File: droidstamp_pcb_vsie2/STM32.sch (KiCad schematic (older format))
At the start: 52 parts, among them P6 CONN_5X2, P8 CONN_12X2, P9 CONN_12X2, Q2 BS170F, Q3 BS170F, Q4 BS170F, Q5 BS170F, Q6 BS170F, Q7 BS170F, Q8 BS170F, Q9 BS170F, U10 STM32F105RC, U11 LT1117CST-3.3, U12 ZXMHC3F381N8, U13 ZXMHC3F381N8, U14 ZXMHC3F381N8, U15 ZXMHC3F381N8, U9 STM32F4_LQFP100, X3 12MHz

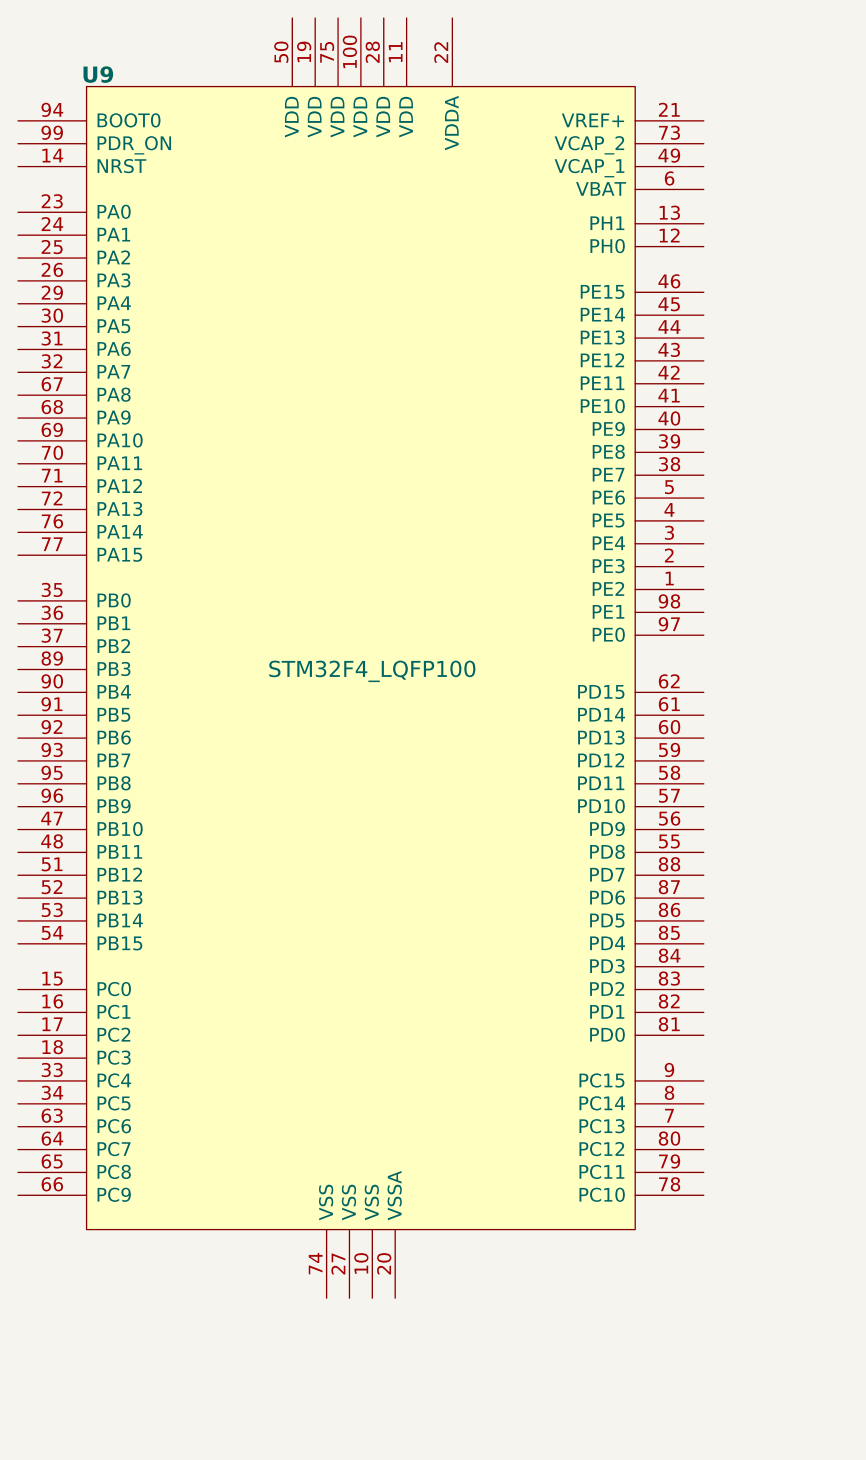
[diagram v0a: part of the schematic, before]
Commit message: sync with las sie_bot_v2
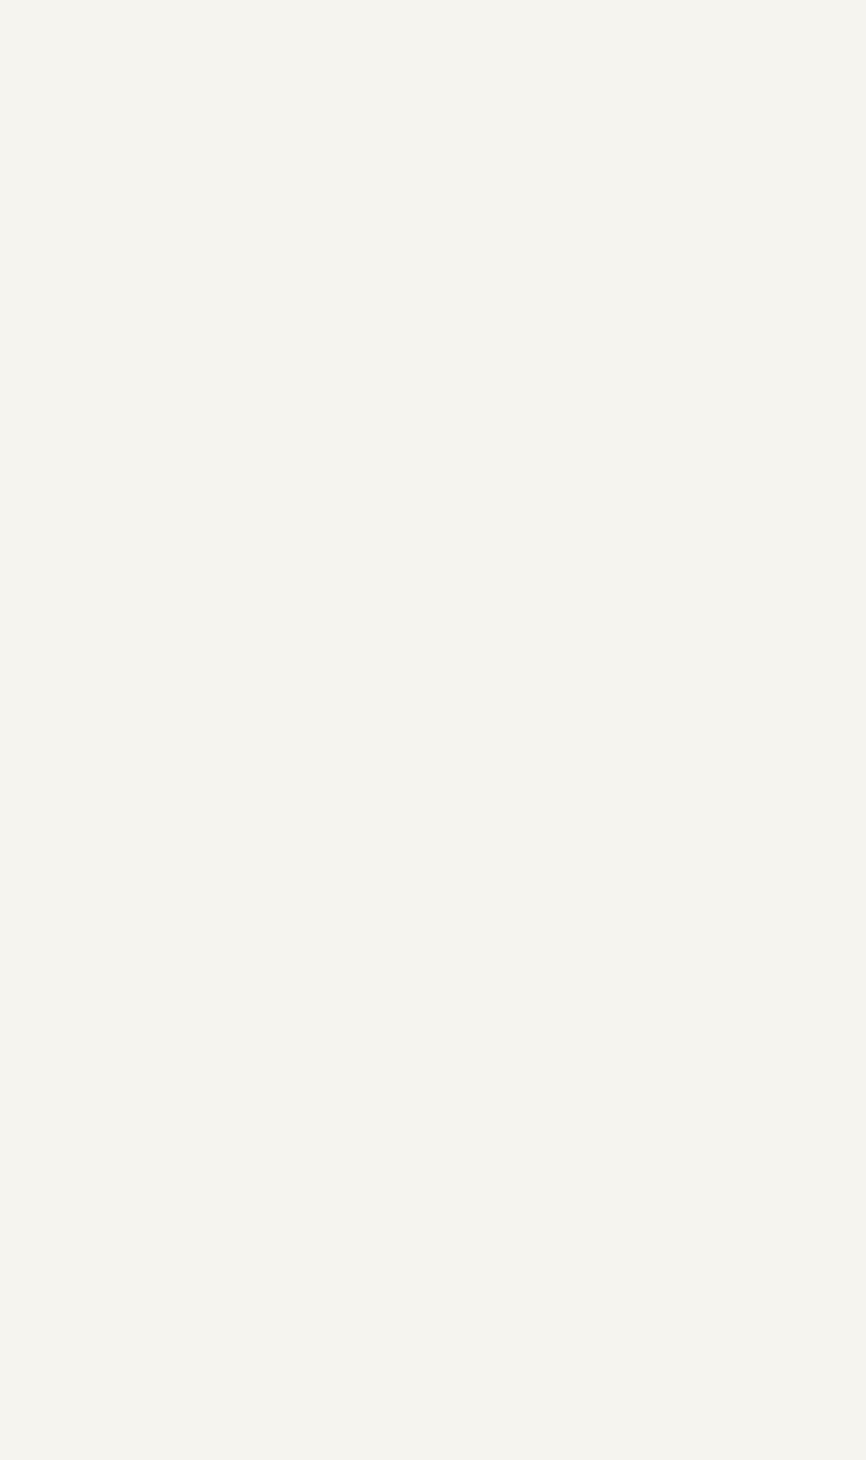
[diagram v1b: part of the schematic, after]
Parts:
- removed U9: STM32F4_LQFP100, TQFP_100, symbol STM32F4_LQFP100
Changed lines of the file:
@@
-EESchema Schematic File Version 2  date Thu 29 Mar 2012 07:34:40 PM COT
+EESchema Schematic File Version 2  date Fri 30 Mar 2012 08:38:46 AM COT
 LIBS:con-jack
 LIBS:adm3101e
@@
 LIBS:lt1117cst
 LIBS:zxmhc3f381n8
-LIBS:stm32f4_lqfp100
 LIBS:i.mx233stamp-cache
 EELAYER 25  0
@@
 $Descr User 12000 10000
 encoding utf-8
-Sheet 4 5
+Sheet 3 5
 Title ""
 Date "30 mar 2012"
@@
 C19, C21 2.2uF para cortex M4\nC19. C21 = Ohms para cortex M3
 $Comp
-L GND #PWR98
+L GND #PWR087
 U 1 1 4F3EDF04
 P 4400 7650
-F 0 "#PWR98" H 4400 7650 30  0001 C CNN
+F 0 "#PWR087" H 4400 7650 30  0001 C CNN
 F 1 "GND" H 4400 7580 30  0001 C CNN
 	1    4400 7650
@@
 $EndComp
 $Comp
-L GND #PWR97
+L GND #PWR088
 U 1 1 4F3EDF01
 P 4200 7650
-F 0 "#PWR97" H 4200 7650 30  0001 C CNN
+F 0 "#PWR088" H 4200 7650 30  0001 C CNN
 F 1 "GND" H 4200 7580 30  0001 C CNN
 	1    4200 7650
@@
 $EndComp
 $Comp
-L 3V3 #PWR104
+L 3V3 #PWR95
 U 1 1 4F3E63FA
 P 6050 8850
-F 0 "#PWR104" H 6050 8950 30  0001 C CNN
+F 0 "#PWR95" H 6050 8950 30  0001 C CNN
 F 1 "3V3" H 6050 8960 30  0000 C CNN
 	1    6050 8850
@@
 $EndComp
 $Comp
-L 3V3 #PWR103
+L 3V3 #PWR94
 U 1 1 4F3E63F9
 P 6050 8750
-F 0 "#PWR103" H 6050 8850 30  0001 C CNN
+F 0 "#PWR94" H 6050 8850 30  0001 C CNN
 F 1 "3V3" H 6050 8860 30  0000 C CNN
 	1    6050 8750
@@
 GND
 $Comp
-L 3V3 #PWR101
+L 3V3 #PWR92
 U 1 1 4F3E4E25
 P 6050 8550
-F 0 "#PWR101" H 6050 8650 30  0001 C CNN
+F 0 "#PWR92" H 6050 8650 30  0001 C CNN
 F 1 "3V3" H 6050 8660 30  0000 C CNN
 	1    6050 8550
@@
 $EndComp
 $Comp
-L 3V3 #PWR102
+L 3V3 #PWR93
 U 1 1 4F3E4E22
 P 6050 8650
-F 0 "#PWR102" H 6050 8750 30  0001 C CNN
+F 0 "#PWR93" H 6050 8750 30  0001 C CNN
 F 1 "3V3" H 6050 8760 30  0000 C CNN
 	1    6050 8650
@@
 $EndComp
 $Comp
-L 3V3 #PWR93
+L 3V3 #PWR84
 U 1 1 4F352D37
 P 2050 6850
-F 0 "#PWR93" H 2050 6950 30  0001 C CNN
+F 0 "#PWR84" H 2050 6950 30  0001 C CNN
 F 1 "3V3" H 2050 6960 30  0000 C CNN
 	1    2050 6850
@@
 I2C1_SDA
 $Comp
-L 3V3 #PWR105
+L 3V3 #PWR96
 U 1 1 4E8A099D
 P 6050 8950
-F 0 "#PWR105" H 6050 9050 30  0001 C CNN
+F 0 "#PWR96" H 6050 9050 30  0001 C CNN
 F 1 "3V3" H 6050 9060 30  0000 C CNN
 	1    6050 8950
@@
 $EndComp
 $Comp
-L 3V3 #PWR94
+L 3V3 #PWR85
 U 1 1 4E8A0997
 P 3700 7900
-F 0 "#PWR94" H 3700 8000 30  0001 C CNN
+F 0 "#PWR85" H 3700 8000 30  0001 C CNN
 F 1 "3V3" H 3700 8010 30  0000 C CNN
 	1    3700 7900
@@
 $EndComp
 $Comp
-L 3V3 #PWR92
+L 3V3 #PWR83
 U 1 1 4E8A0992
 P 1500 7900
-F 0 "#PWR92" H 1500 8000 30  0001 C CNN
+F 0 "#PWR83" H 1500 8000 30  0001 C CNN
 F 1 "3V3" H 1500 8010 30  0000 C CNN
 	1    1500 7900
@@
 $EndComp
 $Comp
-L VDD5V #PWR106
+L VDD5V #PWR089
 U 1 1 4E7B5061
 P 6700 1000
-F 0 "#PWR106" H 6700 1100 30  0001 C CNN
+F 0 "#PWR089" H 6700 1100 30  0001 C CNN
 F 1 "VDD5V" H 6700 1100 30  0000 C CNN
 	1    6700 1000
@@
 $EndComp
 $Comp
-L GND #PWR107
+L GND #PWR090
 U 1 1 4E7B4E89
 P 6700 1650
-F 0 "#PWR107" H 6700 1650 30  0001 C CNN
+F 0 "#PWR090" H 6700 1650 30  0001 C CNN
 F 1 "GND" H 6700 1580 30  0001 C CNN
 	1    6700 1650
@@
 $EndComp
 $Comp
-L GND #PWR111
+L GND #PWR091
 U 1 1 4E7B4E84
 P 8150 1650
-F 0 "#PWR111" H 8150 1650 30  0001 C CNN
+F 0 "#PWR091" H 8150 1650 30  0001 C CNN
 F 1 "GND" H 8150 1580 30  0001 C CNN
 	1    8150 1650
@@
 $EndComp
 $Comp
-L GND #PWR109
+L GND #PWR092
 U 1 1 4E7B44BE
 P 7750 1650
-F 0 "#PWR109" H 7750 1650 30  0001 C CNN
+F 0 "#PWR092" H 7750 1650 30  0001 C CNN
 F 1 "GND" H 7750 1580 30  0001 C CNN
 	1    7750 1650
@@
 $EndComp
 $Comp
-L GND #PWR108
+L GND #PWR093
 U 1 1 4E7B44A2
 P 6900 1250
-F 0 "#PWR108" H 6900 1250 30  0001 C CNN
+F 0 "#PWR093" H 6900 1250 30  0001 C CNN
 F 1 "GND" H 6900 1180 30  0001 C CNN
 	1    6900 1250
@@
 $EndComp
 $Comp
-L 3V3 #PWR110
+L 3V3 #PWR101
 U 1 1 4E7B4482
 P 8150 900
-F 0 "#PWR110" H 8150 1000 30  0001 C CNN
+F 0 "#PWR101" H 8150 1000 30  0001 C CNN
 F 1 "3V3" H 8150 1010 30  0000 C CNN
 	1    8150 900
@@
 $EndComp
 $Comp
-L GND #PWR120
+L GND #PWR094
 U 1 1 4E78C5F4
 P 10800 2850
-F 0 "#PWR120" H 10800 2850 30  0001 C CNN
+F 0 "#PWR094" H 10800 2850 30  0001 C CNN
 F 1 "GND" H 10800 2780 30  0001 C CNN
 	1    10800 2850
@@
 $EndComp
 $Comp
-L 3V3 #PWR113
+L 3V3 #PWR104
 U 1 1 4E78C319
 P 8550 2150
-F 0 "#PWR113" H 8550 2250 30  0001 C CNN
+F 0 "#PWR104" H 8550 2250 30  0001 C CNN
 F 1 "3V3" H 8550 2260 30  0000 C CNN
 	1    8550 2150
@@
 $EndComp
 $Comp
-L GND #PWR100
+L GND #PWR095
 U 1 1 4E78C2ED
 P 5300 7400
-F 0 "#PWR100" H 5300 7400 30  0001 C CNN
+F 0 "#PWR095" H 5300 7400 30  0001 C CNN
 F 1 "GND" H 5300 7330 30  0001 C CNN
 	1    5300 7400
@@
 JTDI
 $Comp
-L 3V3 #PWR96
+L 3V3 #PWR87
 U 1 1 4E78BA06
 P 4150 1100
-F 0 "#PWR96" H 4150 1200 30  0001 C CNN
+F 0 "#PWR87" H 4150 1200 30  0001 C CNN
 F 1 "3V3" H 4150 1210 30  0000 C CNN
 	1    4150 1100
@@
 $EndComp
 $Comp
-L 3V3 #PWR112
+L 3V3 #PWR103
 U 1 1 4E2A2E11
 P 8350 2150
-F 0 "#PWR112" H 8350 2250 30  0001 C CNN
+F 0 "#PWR103" H 8350 2250 30  0001 C CNN
 F 1 "3V3" H 8350 2260 30  0000 C CNN
 	1    8350 2150
@@
 $EndComp
 $Comp
-L 3V3 #PWR115
+L 3V3 #PWR106
 U 1 1 4E2A2E03
 P 8750 1000
-F 0 "#PWR115" H 8750 1100 30  0001 C CNN
+F 0 "#PWR106" H 8750 1100 30  0001 C CNN
 F 1 "3V3" H 8750 1110 30  0000 C CNN
 	1    8750 1000
@@
 $EndComp
 $Comp
-L 3V3 #PWR99
+L 3V3 #PWR90
 U 1 1 4E2A2DF0
 P 4700 1150
-F 0 "#PWR99" H 4700 1250 30  0001 C CNN
+F 0 "#PWR90" H 4700 1250 30  0001 C CNN
 F 1 "3V3" H 4700 1260 30  0000 C CNN
 	1    4700 1150
@@
 $EndComp
 $Comp
-L GND #PWR119
+L GND #PWR096
 U 1 1 4E188E4E
 P 10550 1500
-F 0 "#PWR119" H 10550 1500 30  0001 C CNN
+F 0 "#PWR096" H 10550 1500 30  0001 C CNN
 F 1 "GND" H 10550 1430 30  0001 C CNN
 	1    10550 1500
@@
 FP1
 $Comp
-L GND #PWR116
+L GND #PWR097
 U 1 1 4E186DEB
 P 9250 1500
-F 0 "#PWR116" H 9250 1500 30  0001 C CNN
+F 0 "#PWR097" H 9250 1500 30  0001 C CNN
 F 1 "GND" H 9250 1430 30  0001 C CNN
 	1    9250 1500
@@
 $EndComp
 $Comp
-L GND #PWR114
+L GND #PWR098
 U 1 1 4E07869F
 P 8550 2800
-F 0 "#PWR114" H 8550 2800 30  0001 C CNN
+F 0 "#PWR098" H 8550 2800 30  0001 C CNN
 F 1 "GND" H 8550 2730 30  0001 C CNN
 	1    8550 2800
@@
 $EndComp
 $Comp
-L GND #PWR95
+L GND #PWR099
 U 1 1 4DCDB18D
 P 4000 7400
-F 0 "#PWR95" H 4000 7400 30  0001 C CNN
+F 0 "#PWR099" H 4000 7400 30  0001 C CNN
 F 1 "GND" H 4000 7330 30  0001 C CNN
 	1    4000 7400
@@
 $EndComp
 $Comp
-L GND #PWR117
+L GND #PWR0100
 U 1 1 4DCDB183
 P 9650 2800
-F 0 "#PWR117" H 9650 2800 30  0001 C CNN
+F 0 "#PWR0100" H 9650 2800 30  0001 C CNN
 F 1 "GND" H 9650 2730 30  0001 C CNN
 	1    9650 2800
@@
 NRST
 $Comp
-L GND #PWR91
+L GND #PWR0101
 U 1 1 4DCDB180
 P 700 2050
-F 0 "#PWR91" H 700 2050 30  0001 C CNN
+F 0 "#PWR0101" H 700 2050 30  0001 C CNN
 F 1 "GND" H 700 1980 30  0001 C CNN
 	1    700  2050
@@
 BOOT0
 $Comp
-L GND #PWR118
+L GND #PWR0102
 U 1 1 4DCDB17D
 P 10400 2850
-F 0 "#PWR118" H 10400 2850 30  0001 C CNN
+F 0 "#PWR0102" H 10400 2850 30  0001 C CNN
 F 1 "GND" H 10400 2780 30  0001 C CNN
 	1    10400 2850
@@
 	0    1    1    0
 $EndComp
-$Comp
-L STM32F4_LQFP100 U9
-U 1 1 4F750C24
-P -2750 950
-F 0 "U9" H -4000 3350 70  0000 C CNB
-F 1 "STM32F4_LQFP100" H -2800 750 70  0000 C CNN
-F 2 "TQFP_100" H -2750 950 60  0001 C CNN
-	1    -2750 950
-	1    0    0    -1
-$EndComp
 $EndSCHEMATC
